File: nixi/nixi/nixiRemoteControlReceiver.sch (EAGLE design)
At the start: 17 parts, among them IC1 7805L, IC2 4081D, IC3 40106D, K1 TXD2-1.5V, K2 TXD2-1.5V, T1 2N3904, T2 2N3904

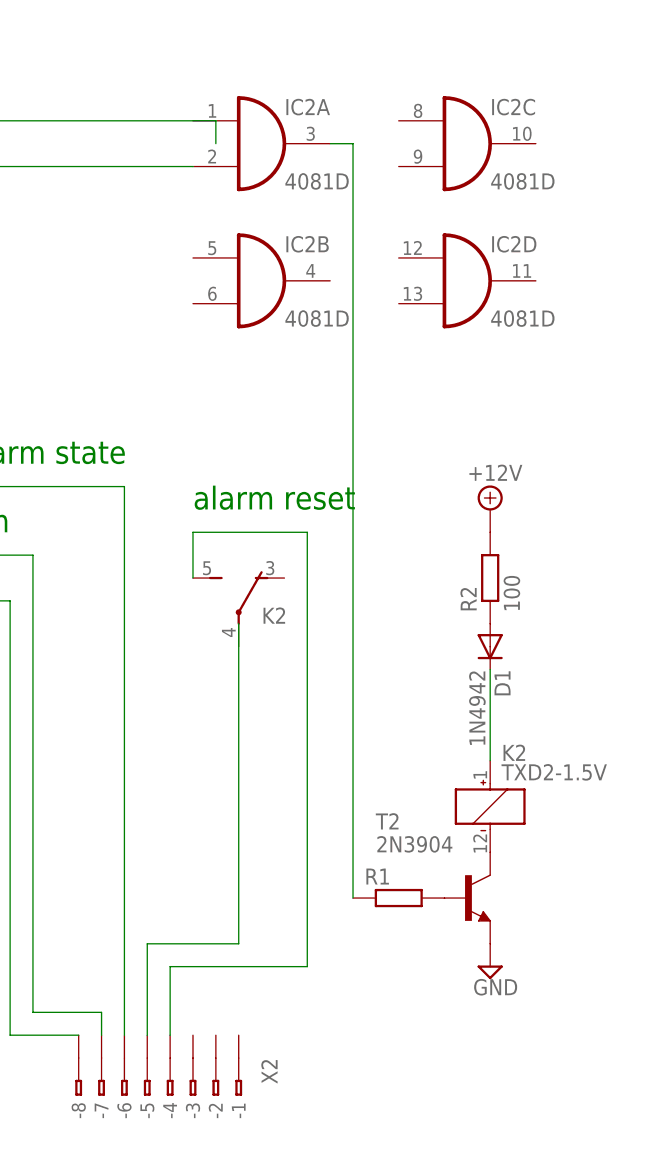
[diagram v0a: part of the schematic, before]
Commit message: reg save
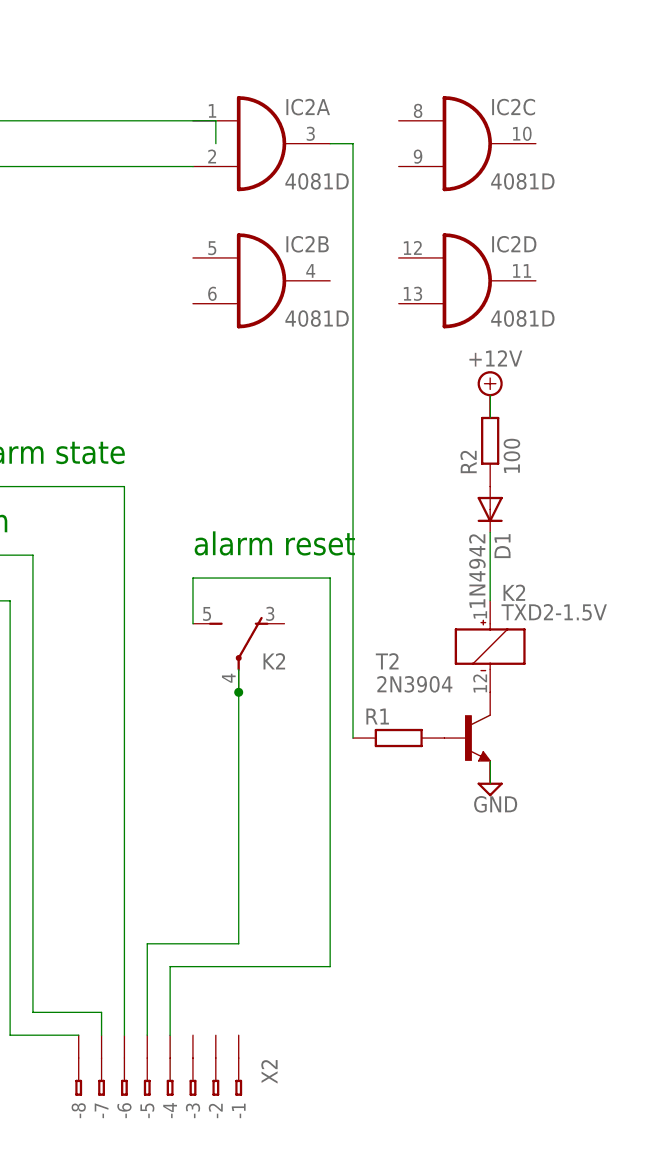
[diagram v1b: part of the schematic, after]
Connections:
- net N$8: now also K2G$1.P
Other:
- moved on the sheet: D1, K2, R1, R2, T2
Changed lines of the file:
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@@
 <text x="111.76" y="38.1" size="2.54" layer="91">white</text>
 <text x="139.7" y="45.72" size="2.54" layer="91">alarm state</text>
-<text x="165.1" y="40.64" size="2.54" layer="91">alarm reset</text>
+<text x="165.1" y="35.56" size="2.54" layer="91">alarm reset</text>
 <text x="127" y="38.1" size="2.54" layer="91">170 V pwm</text>
 <text x="124.46" y="-7.62" size="2.54" layer="91">blue leds</text>
@@
 <instances>
 <instance part="T1" gate="G1" x="66.04" y="68.58"/>
-<instance part="T2" gate="G1" x="195.58" y="-2.54"/>
+<instance part="T2" gate="G1" x="195.58" y="15.24"/>
 <instance part="IC1" gate="A1" x="71.12" y="27.94"/>
 <instance part="C2" gate="G$1" x="68.58" y="60.96"/>
 <instance part="C3" gate="G$1" x="88.9" y="20.32"/>
-<instance part="R1" gate="G$1" x="187.96" y="-2.54"/>
-<instance part="D1" gate="1" x="198.12" y="25.4" rot="R270"/>
+<instance part="R1" gate="G$1" x="187.96" y="15.24"/>
+<instance part="D1" gate="1" x="198.12" y="40.64" rot="R270"/>
 <instance part="K1" gate="_" x="111.76" y="20.32"/>
 <instance part="K1" gate="G$1" x="129.54" y="25.4"/>
 <instance part="K1" gate="G$2" x="129.54" y="12.7"/>
-<instance part="K2" gate="_" x="198.12" y="7.62"/>
-<instance part="K2" gate="G$1" x="170.18" y="27.94"/>
+<instance part="K2" gate="_" x="198.12" y="25.4"/>
+<instance part="K2" gate="G$1" x="170.18" y="22.86"/>
 <instance part="IC2" gate="A" x="172.72" y="81.28"/>
 <instance part="IC2" gate="B" x="172.72" y="66.04"/>
@@
 <instance part="SUPPLY3" gate="GND" x="78.74" y="7.62"/>
 <instance part="C4" gate="G$1" x="58.42" y="20.32"/>
-<instance part="SUPPLY5" gate="+12V" x="198.12" y="40.64"/>
-<instance part="R2" gate="G$1" x="198.12" y="33.02" rot="R90"/>
-<instance part="SUPPLY6" gate="GND" x="198.12" y="-10.16"/>
+<instance part="SUPPLY5" gate="+12V" x="198.12" y="53.34"/>
+<instance part="R2" gate="G$1" x="198.12" y="48.26" rot="R90"/>
+<instance part="SUPPLY6" gate="GND" x="198.12" y="10.16"/>
 <instance part="SUPPLY7" gate="+5V" x="68.58" y="76.2"/>
 <instance part="R3" gate="G$1" x="86.36" y="60.96" rot="R90"/>
@@
 <pinref part="SUPPLY5" gate="+12V" pin="+12V"/>
 <pinref part="R2" gate="G$1" pin="2"/>
+<wire x1="198.12" y1="53.34" x2="198.12" y2="50.8" width="0.1524" layer="91"/>
 </segment>
 </net>
@@
 <pinref part="T2" gate="G1" pin="E"/>
 <pinref part="SUPPLY6" gate="GND" pin="GND"/>
+<wire x1="198.12" y1="12.7" x2="198.12" y2="10.16" width="0.1524" layer="91"/>
 </segment>
 <segment>
@@
 <net name="N$7" class="0">
 <segment>
-<wire x1="177.8" y1="38.1" x2="177.8" y2="-10.16" width="0.1524" layer="91"/>
-<wire x1="177.8" y1="-10.16" x2="162.56" y2="-10.16" width="0.1524" layer="91"/>
+<wire x1="180.34" y1="33.02" x2="180.34" y2="-10.16" width="0.1524" layer="91"/>
+<wire x1="180.34" y1="-10.16" x2="162.56" y2="-10.16" width="0.1524" layer="91"/>
 <pinref part="X2" gate="G$1" pin="B-4"/>
 <wire x1="162.56" y1="-10.16" x2="162.56" y2="-17.78" width="0.1524" layer="91"/>
-<wire x1="177.8" y1="38.1" x2="165.1" y2="38.1" width="0.1524" layer="91"/>
+<wire x1="180.34" y1="33.02" x2="165.1" y2="33.02" width="0.1524" layer="91"/>
 <pinref part="K2" gate="G$1" pin="S"/>
-<wire x1="165.1" y1="38.1" x2="165.1" y2="33.02" width="0.1524" layer="91"/>
+<wire x1="165.1" y1="33.02" x2="165.1" y2="27.94" width="0.1524" layer="91"/>
 </segment>
 </net>
@@
 <wire x1="160.02" y1="-7.62" x2="160.02" y2="-17.78" width="0.1524" layer="91"/>
 <wire x1="160.02" y1="-7.62" x2="170.18" y2="-7.62" width="0.1524" layer="91"/>
-<wire x1="170.18" y1="-7.62" x2="170.18" y2="27.94" width="0.1524" layer="91"/>
+<wire x1="170.18" y1="-7.62" x2="170.18" y2="20.32" width="0.1524" layer="91"/>
+<pinref part="K2" gate="G$1" pin="P"/>
+<wire x1="170.18" y1="20.32" x2="170.18" y2="22.86" width="0.1524" layer="91"/>
+<junction x="170.18" y="20.32"/>
 </segment>
 </net>
@@
 <pinref part="D1" gate="1" pin="C"/>
 <pinref part="K2" gate="_" pin="+"/>
-<wire x1="198.12" y1="22.86" x2="198.12" y2="12.7" width="0.1524" layer="91"/>
+<wire x1="198.12" y1="38.1" x2="198.12" y2="30.48" width="0.1524" layer="91"/>
 </segment>
 </net>
@@
 <wire x1="180.34" y1="81.28" x2="182.88" y2="81.28" width="0.1524" layer="91"/>
 <pinref part="R1" gate="G$1" pin="1"/>
-<wire x1="182.88" y1="81.28" x2="182.88" y2="-2.54" width="0.1524" layer="91"/>
-</segment>
-</net>
+<wire x1="182.88" y1="81.28" x2="182.88" y2="15.24" width="0.1524" layer="91"/>
+</segment>
+</net>
